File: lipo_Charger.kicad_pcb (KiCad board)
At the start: 4 copper layers, 98 parts, among them J1 XT60PW-M, J3 balance_plug_4s, J4 Conn_01x05, J5 Conn_01x04, J7 Conn_01x07, Q1 NX7002AK_215(nch low power), Q2 NVTFS010N10MCLTAG(high power), Q3 NVTFS010N10MCLTAG(high power), Q4 NVTFS010N10MCLTAG(high power), Q5 NVTFS010N10MCLTAG(high power), Q6 NX7002AK_215(nch low power), Q7 NX7002AK_215(nch low power), Q8 NX7002AK_215(nch low power), U1 BQ25703ARSNR

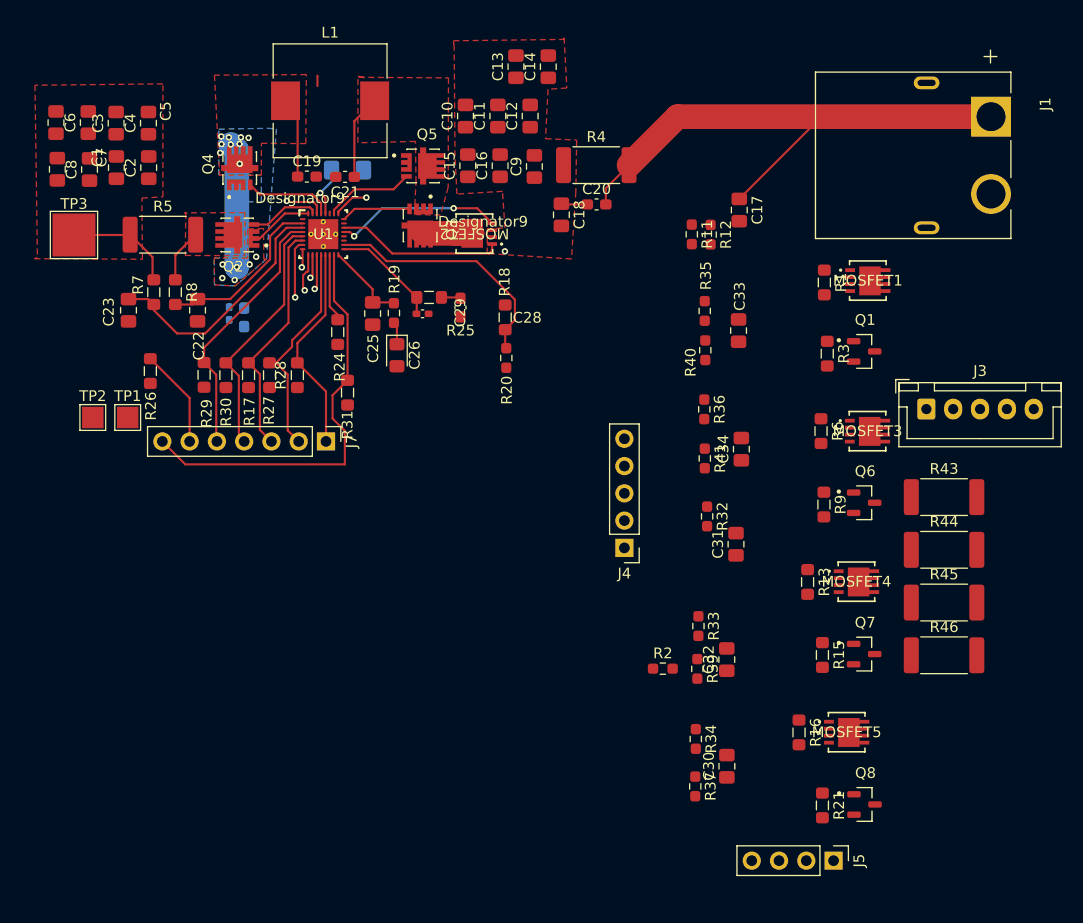
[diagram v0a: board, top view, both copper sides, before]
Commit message: done everything need to check before ordering once
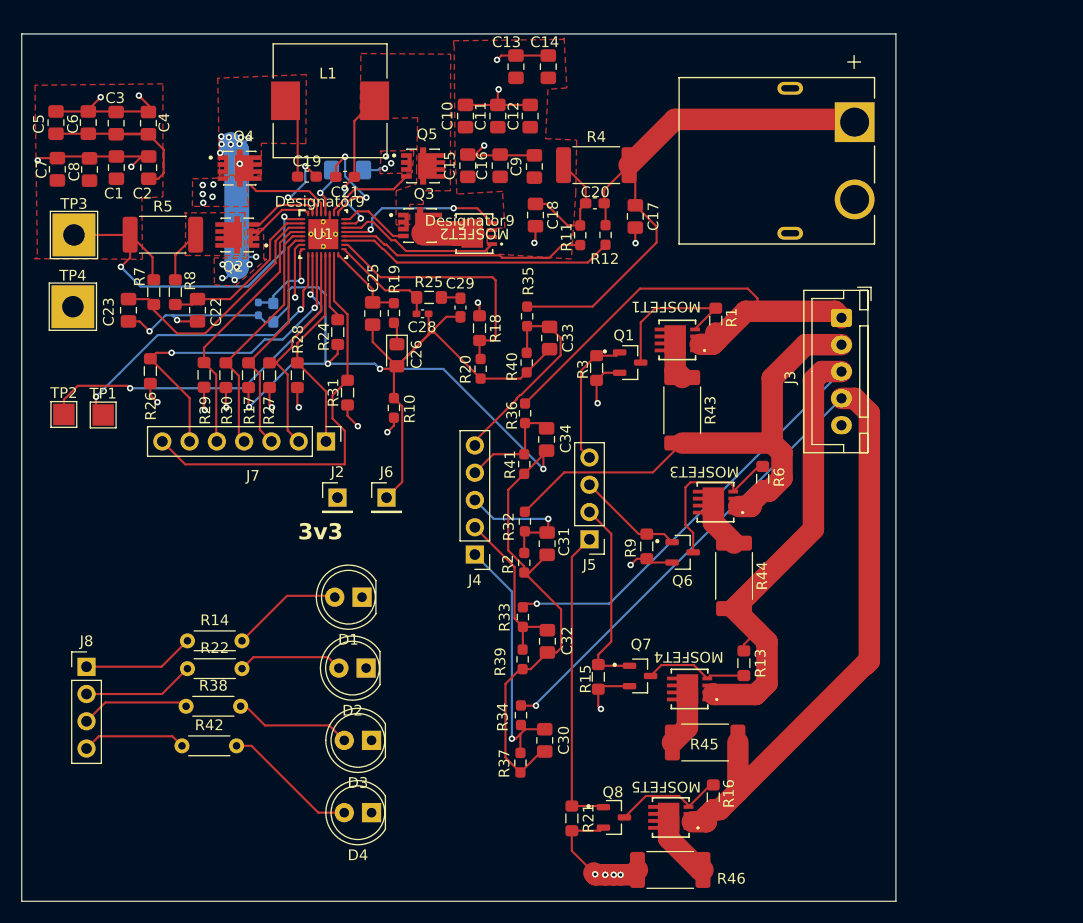
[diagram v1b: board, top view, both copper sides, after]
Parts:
- added D1: LED, LED_THT:LED_D5.0mm, F.Cu at (127.6, 106.4)
- added D2: LED, LED_THT:LED_D5.0mm, F.Cu at (128.0, 113.0)
- added D3: LED, LED_THT:LED_D5.0mm, F.Cu at (128.5, 119.8)
- added D4: LED, LED_THT:LED_D5.0mm, F.Cu at (128.5, 126.5)
- added J2: Conn_01x01, Connector_PinHeader_2.54mm:PinHeader_1x01_P2.54mm_Vertical, F.Cu at (125.3, 97.2)
- added J6: Conn_01x01, Connector_PinHeader_2.54mm:PinHeader_1x01_P2.54mm_Vertical, F.Cu at (129.9, 97.2)
- added J8: Conn_01x04, Connector_PinHeader_2.54mm:PinHeader_1x04_P2.54mm_Vertical, F.Cu at (102.0, 112.9)
- added R10: 0ohm, Resistor_SMD:R_0603_1608Metric_Pad0.98x0.95mm_HandSolder, F.Cu at (130.6, 88.8)
- added R14: R, Resistor_THT:R_Axial_DIN0204_L3.6mm_D1.6mm_P5.08mm_Horizontal, F.Cu at (111.4, 110.5)
- added R22: R, Resistor_THT:R_Axial_DIN0204_L3.6mm_D1.6mm_P5.08mm_Horizontal, F.Cu at (111.4, 113.1)
- added R38: R, Resistor_THT:R_Axial_DIN0204_L3.6mm_D1.6mm_P5.08mm_Horizontal, F.Cu at (111.3, 116.6)
- added R42: R, Resistor_THT:R_Axial_DIN0204_L3.6mm_D1.6mm_P5.08mm_Horizontal, F.Cu at (110.9, 120.3)
- added TP4: TestPoint, TestPoint:TestPoint_THTPad_4.0x4.0mm_Drill2.0mm, F.Cu at (100.7, 79.4)
- TP3: footprint TestPoint:TestPoint_Pad_4.0x4.0mm -> TestPoint:TestPoint_THTPad_4.0x4.0mm_Drill2.0mm
- moved J5 37.6 mm to (148.8, 101.0), turned to 180 degrees
- moved R46 32.4 mm to (156.3, 131.8), turned to 180 degrees
- moved R45 25.8 mm to (159.6, 120.0)
- moved R43 25.7 mm to (157.5, 89.0), turned to -90 degrees
- moved Q8 23.4 mm to (151.1, 126.9)
- moved R21 23.4 mm to (147.2, 127.0)
- moved Q1 21.8 mm to (152.6, 84.6)
- moved R3 21.5 mm to (149.5, 85.1)
- moved Q7 21.0 mm to (153.5, 113.8)
- moved R15 21.0 mm to (149.6, 113.8)
- moved R44 19.7 mm to (162.3, 104.4), turned to -90 degrees
- moved MOSFET1 18.6 mm to (157.0, 82.5), turned to 180 degrees
- moved MOSFET4 18.5 mm to (158.1, 115.0), turned to 180 degrees
- moved MOSFET5 18.2 mm to (156.4, 126.9), turned to 180 degrees
- moved C34 18.2 mm to (144.8, 91.7)
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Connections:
- C24 pad 2: GNDA -> GND
- C30 pad 1: GND -> GNDA
- R37 pad 2: GND -> GNDA
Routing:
- net GNDA: track 0.00 -> 161.8 mm, vias 0 -> 6
- net /CELL_1S: track 0.00 -> 95.6 mm, vias 0 -> 1
- net /CELL_2S: track 0.00 -> 82.1 mm, vias 0 -> 1
- net GND: track 0.00 -> 80.3 mm, vias 0 -> 25
- net /CELL_3S: track 0.00 -> 48.5 mm
- net /CELL_4S: track 0.00 -> 43.6 mm
- net +24V: track 10.4 -> 53.5 mm, vias 0 -> 2
- net Net-(U1-PSYS): track 2.22 -> 34.6 mm, vias 1 -> 2
- net Net-(J5-Pin_1): track 0.00 -> 28.5 mm
- net Net-(U1-IBAT): track 3.61 -> 29.8 mm, vias 1 -> 2
- net Net-(U1-SRN): track 0.00 -> 25.9 mm
- net /CELL_1S_adc: track 0.00 -> 24.3 mm, vias 0 -> 1
- net Net-(U1-SRP): track 0.00 -> 24.0 mm
- net /BAT_adc: track 0.00 -> 19.4 mm
- net /PROCHOT_N: track 12.5 -> 31.5 mm, vias 1 -> 2
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- added copper zone on F.Cu, net GND
- added copper zone on In2.Cu, net VDDA
- removed copper zone on B.Cu, net (none)
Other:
- board outline added: 81.4 x 80.8 mm
- board text added: "3v3"
